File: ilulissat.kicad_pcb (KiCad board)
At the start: 2 copper layers, 25.4 x 25.4 mm, 31 parts, among them J1 Conn_01x06, SW1 ~RST~, SW2 USR, U1 EFR32MG21x, U2 HDC2080, Y1 32.768Khz, Y2 38.4Mhz

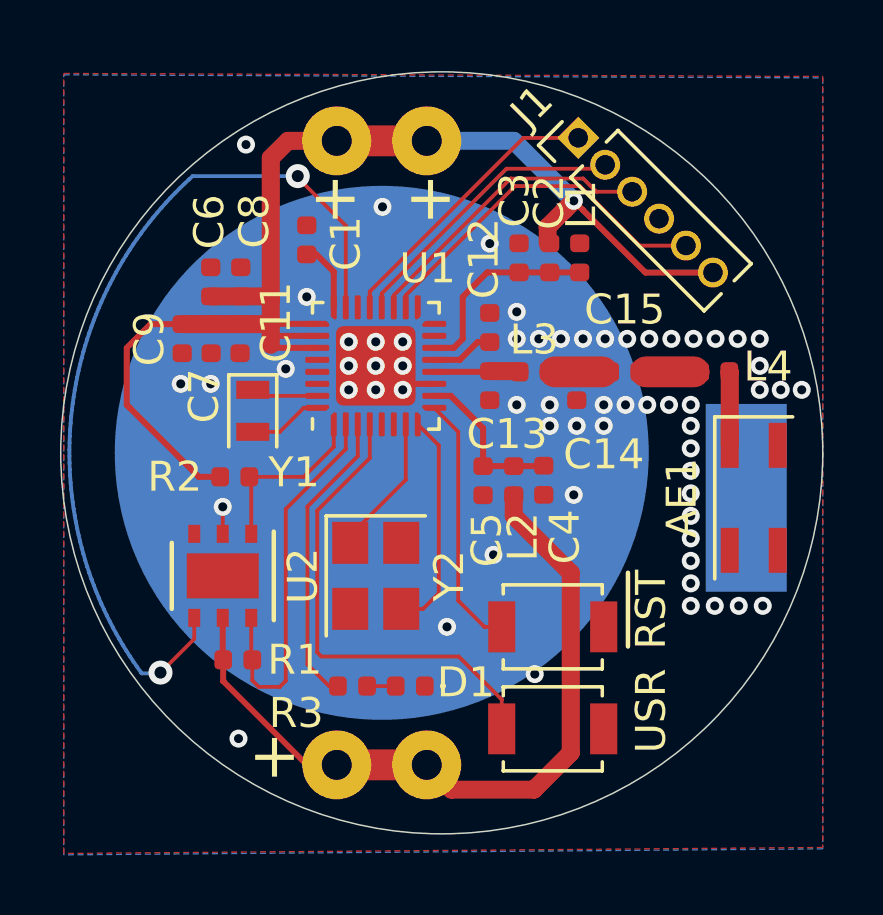
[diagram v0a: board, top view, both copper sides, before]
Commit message: Rev1
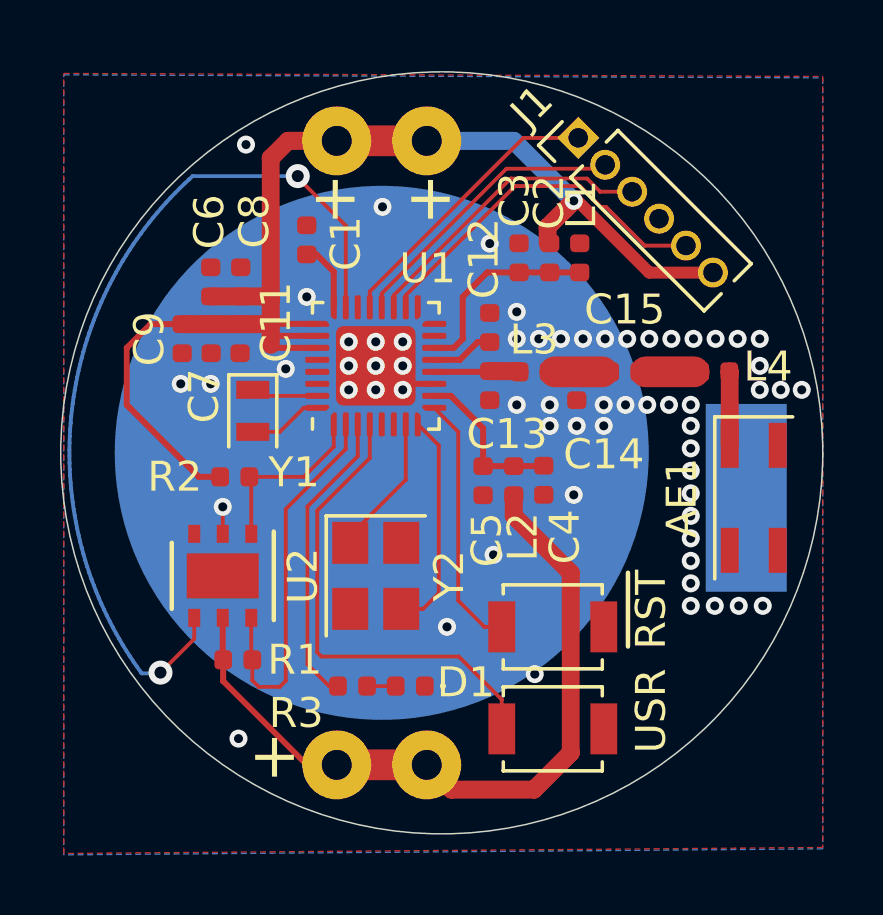
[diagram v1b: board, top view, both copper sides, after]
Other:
- net class Default: clearance 0.2 -> 0.127; trace_width 0.25 -> 0.2
- rule trace_clearance: 0.2 -> 0.127
